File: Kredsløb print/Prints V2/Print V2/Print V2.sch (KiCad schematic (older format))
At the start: 79 parts, among them J1 Conn_01x01_Male, J10 Conn_01x01_Male, J11 Conn_01x01_Male, J12 Conn_01x01_Male, J13 Conn_01x01_Male, J14 Conn_01x01_Male, J15 Conn_01x01_Male, J16 Conn_01x01_Male, J17 Conn_01x01_Male, J18 Conn_01x01_Male, J19 Conn_01x01_Male, J2 Conn_01x01_Male, J20 Conn_01x01_Male, J21 Conn_01x01_Male, J22 Conn_01x01_Male, J23 Conn_01x01_Male, J24 Conn_01x01_Male, J25 Conn_01x01_Male, J26 Conn_01x01_Male, J27 Conn_01x01_Male, J28 Conn_01x01_Male, J29 Conn_01x01_Male, J3 Conn_01x01_Male, J30 Conn_01x01_Male, J31 Conn_01x01_Male, J32 Conn_01x01_Male, J33 Conn_01x01, J34 Conn_01x01, J4 Conn_01x01_Male, J5 Conn_01x01_Male, J6 Conn_01x01_Male, J7 Conn_01x01_Male, J8 Conn_01x01_Male, J9 Conn_01x01_Male, Q1 BC547, Q10 TIP120, Q11 TIP127, Q12 TIP120, Q13 TIP127, Q14 TIP120, Q15 BC547, Q16 BC547, Q17 BC547, Q18 TIP127, Q19 TIP120, Q2 BC547, Q20 BC547, Q21 TIP127, Q22 TIP120, Q23 TIP120, Q24 TIP120, Q25 TIP127, Q26 TIP120, Q27 TIP127, Q28 TIP120, Q3 BC547, Q4 TIP127, Q5 TIP120, Q6 BC547, Q7 TIP127, Q8 TIP120, Q9 TIP120, U1 LM7805_TO220, U2 esp32, U3 4049

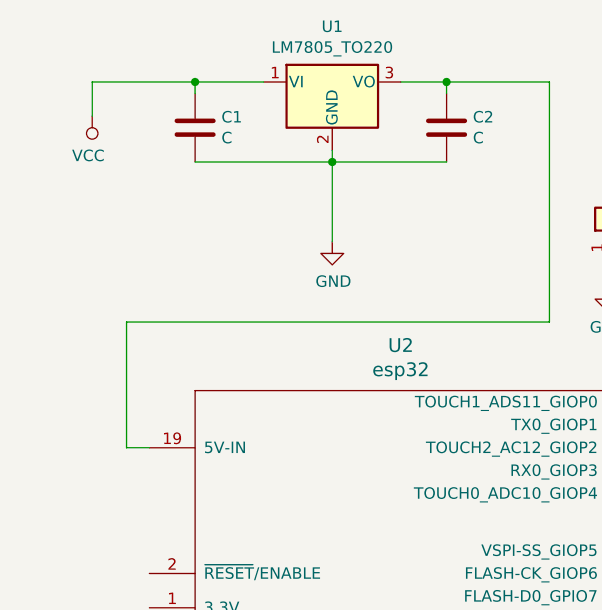
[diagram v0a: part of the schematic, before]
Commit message: stuff
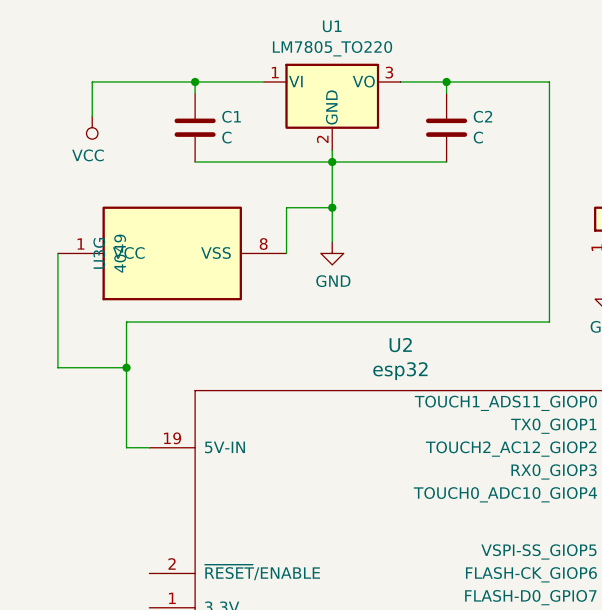
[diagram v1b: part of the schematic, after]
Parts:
- added unit 7 of U3
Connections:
- net GND: now also U3.8 (VSS)
- net at C2.1, U1.3 (VO), U2.19 (5V-IN): now also U3.1 (VCC)
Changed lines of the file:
@@
 	2800 1750 950  1750
 Wire Wire Line
-	950  1750 950  2300
+	950  1750 950  1950
 Connection ~ 2350 700
 Wire Wire Line
 	950  2300 1050 2300
 Wire Wire Line
-	1850 1400 1850 1050
+	1850 1400 1850 1250
 $Comp
 L power:GND #PWR0111
@@
 Wire Wire Line
 	4700 2400 4700 3850
+Wire Wire Line
+	1650 1450 1650 1250
+Wire Wire Line
+	1650 1250 1850 1250
+Connection ~ 1850 1250
+Wire Wire Line
+	1850 1250 1850 1050
+Wire Wire Line
+	650  1450 650  1950
+Wire Wire Line
+	650  1950 950  1950
+Connection ~ 950  1950
+Wire Wire Line
+	950  1950 950  2300
+$Comp
+L 4xxx:4049 U3
+U 7 1 5CB3F75A
+P 1150 1450
+F 0 "U3" H 1150 1767 50  0000 C CNN
+F 1 "4049" H 1150 1676 50  0000 C CNN
+F 2 "Package_DIP:DIP-16_W7.62mm_LongPads" H 1150 1450 50  0001 C CNN
+F 3 "http://www.intersil.com/content/dam/intersil/documents/cd40/cd4049ubms.pdf" H 1150 1450 50  0001 C CNN
+	7    1150 1450
+	0    -1   -1   0
+$EndComp
 $EndSCHEMATC
